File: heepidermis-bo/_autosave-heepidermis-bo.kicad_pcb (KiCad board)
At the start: 4 copper layers, 85.7 x 54 mm, 40 parts, among them J1 Conn_01x03, J10 Conn_Boaxial, J11 Conn_Boaxial, J12 Conn_01x03, J13 Conn_01x03, J14 Conn_01x03, J15 Conn_02x16_Odd_Even, J17 Conn_02x10_Odd_Even, J18 Conn_01x03, J19 Conn_01x03, J2 5025983393, J20 Conn_01x03, J21 Conn_01x03, J22 Conn_01x03, J23 Conn_02x29_Top_Bottom, J5 Conn_01x03, J6 Conn_01x03, J7 Conn_01x03, J8 Conn_01x03, J9 Conn_Boaxial, SW1 SW_Push

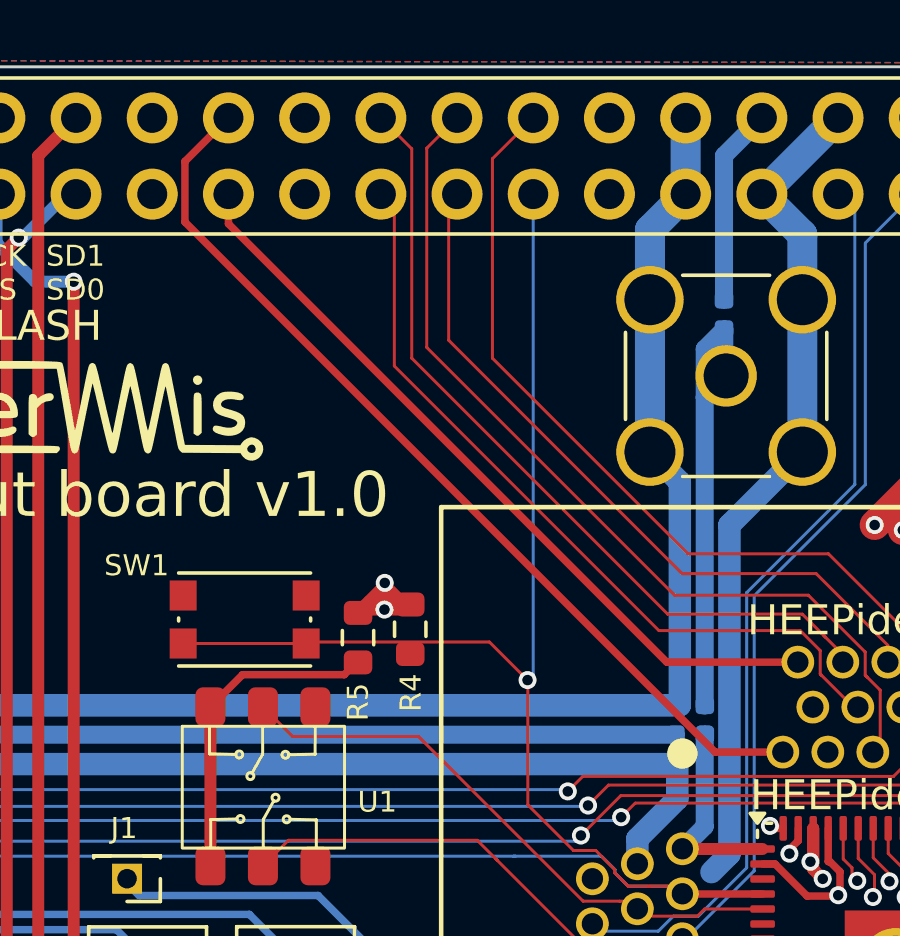
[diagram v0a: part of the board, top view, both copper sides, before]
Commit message: Almost done adding footprint of qfn64
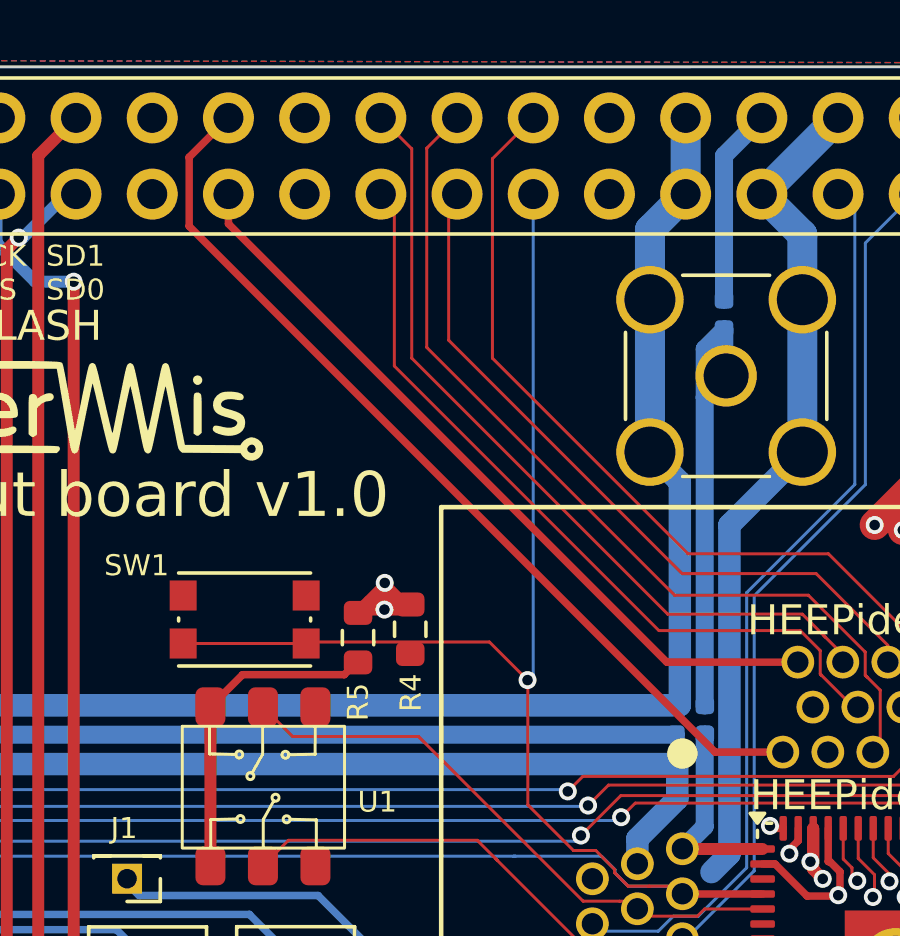
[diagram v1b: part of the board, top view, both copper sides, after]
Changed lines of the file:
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@@
 		)
 		(fp_text user "${REFERENCE}"
-			(at 0.635 1.27 360)
+			(at 0.635 1.27 0)
 			(layer "F.Fab")
 			(effects
@@
 		)
 		(fp_text user "${REFERENCE}"
-			(at 1.27 39.37 360)
+			(at 1.27 39.37 0)
 			(layer "F.Fab")
 			(effects
@@
 		(tags "capacitor")
 		(property "Reference" "C3"
-			(at 0.08 -1.14 360)
+			(at 0.08 -1.14 0)
 			(layer "F.SilkS")
 			(effects
@@
 		)
 		(property "Value" "100n"
-			(at 0 1.43 360)
+			(at 0 1.43 0)
 			(layer "F.Fab")
 			(effects
@@
 		)
 		(fp_text user "${REFERENCE}"
-			(at 0 0 360)
+			(at 0 0 0)
 			(layer "F.Fab")
 			(effects
@@
 		(tags "capacitor")
 		(property "Reference" "C2"
-			(at 2.62 -0.05 360)
+			(at 2.62 -0.05 0)
 			(layer "F.SilkS")
 			(effects
@@
 		)
 		(property "Value" "100n"
-			(at 0 1.43 360)
+			(at 0 1.43 0)
 			(layer "F.Fab")
 			(effects
@@
 		)
 		(fp_text user "${REFERENCE}"
-			(at 0 0 360)
+			(at 0 0 0)
 			(layer "F.Fab")
 			(effects
@@
 		)
 		(fp_text user "${REFERENCE}"
-			(at 0.635 1.27 360)
+			(at 0.635 1.27 0)
 			(layer "F.Fab")
 			(effects
@@
 		(at 104.94 83.36)
 		(property "Reference" "G***"
-			(at 0 0 360)
+			(at 0 0 0)
 			(layer "F.SilkS")
 			(hide yes)
@@
 		)
 		(property "Value" "LOGO"
-			(at 0.75 0 360)
+			(at 0.75 0 0)
 			(layer "F.SilkS")
 			(hide yes)
@@
 		)
 		(property "Footprint" ""
-			(at 0 0 360)
+			(at 0 0 0)
 			(layer "F.Fab")
 			(hide yes)
@@
 		)
 		(property "Datasheet" ""
-			(at 0 0 360)
+			(at 0 0 0)
 			(layer "F.Fab")
 			(hide yes)
@@
 		)
 		(property "Description" ""
-			(at 0 0 360)
+			(at 0 0 0)
 			(layer "F.Fab")
 			(hide yes)
@@
 		(tags "tactile switch kmr2")
 		(property "Reference" "SW1"
-			(at 3.6 1.8 360)
+			(at 3.6 1.8 0)
 			(layer "F.SilkS")
 			(effects
@@
 		)
 		(property "Value" "SW_Push"
-			(at 0 2.55 360)
+			(at 0 2.55 0)
 			(layer "F.Fab")
 			(effects
@@
 		)
 		(fp_text user "${REFERENCE}"
-			(at 0 -2.45 360)
+			(at 0 -2.45 0)
 			(layer "F.Fab")
 			(effects
@@
 	)
 	(segment
-		(start 113.25 74.01)
+		(start 113.39 73.87)
 		(end 114.7 72.56)
 		(width 0.25)
@@
 	)
 	(segment
-		(start 113.25 76.03)
-		(end 113.25 74.01)
+		(start 130.920499 93.700499)
+		(end 113.39 76.17)
 		(width 0.25)
 		(layer "F.Cu")
@@
 	)
 	(segment
-		(start 133.1925 96.2425)
-		(end 132.8325 96.2425)
+		(start 113.39 76.17)
+		(end 113.39 73.87)
 		(width 0.25)
 		(layer "F.Cu")
@@
 	)
 	(segment
-		(start 133.18 93.700499)
-		(end 130.920499 93.700499)
+		(start 133.1925 96.2425)
+		(end 132.8325 96.2425)
 		(width 0.25)
 		(layer "F.Cu")
@@
 	)
 	(segment
-		(start 130.920499 93.700499)
-		(end 113.25 76.03)
+		(start 133.18 93.700499)
+		(end 130.920499 93.700499)
 		(width 0.25)
 		(layer "F.Cu")
